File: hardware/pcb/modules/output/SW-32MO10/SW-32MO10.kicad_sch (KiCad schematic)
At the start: 35 parts, among them Q1 NTF2955, Q2 DMN2041L, Q3 DMN2041L, T1 42TL004-RC, U1 SW-32MO, U2 TLV272IS-13

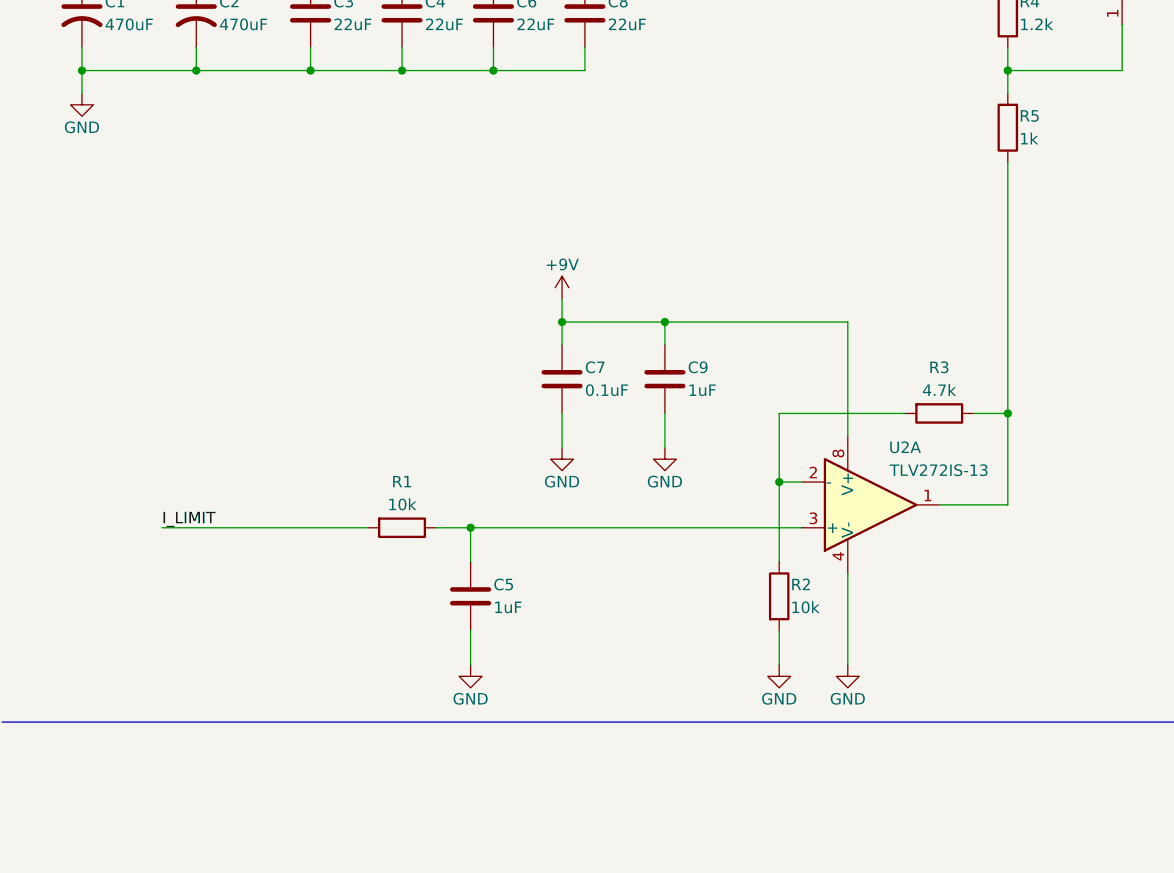
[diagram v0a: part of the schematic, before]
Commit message: update pdf
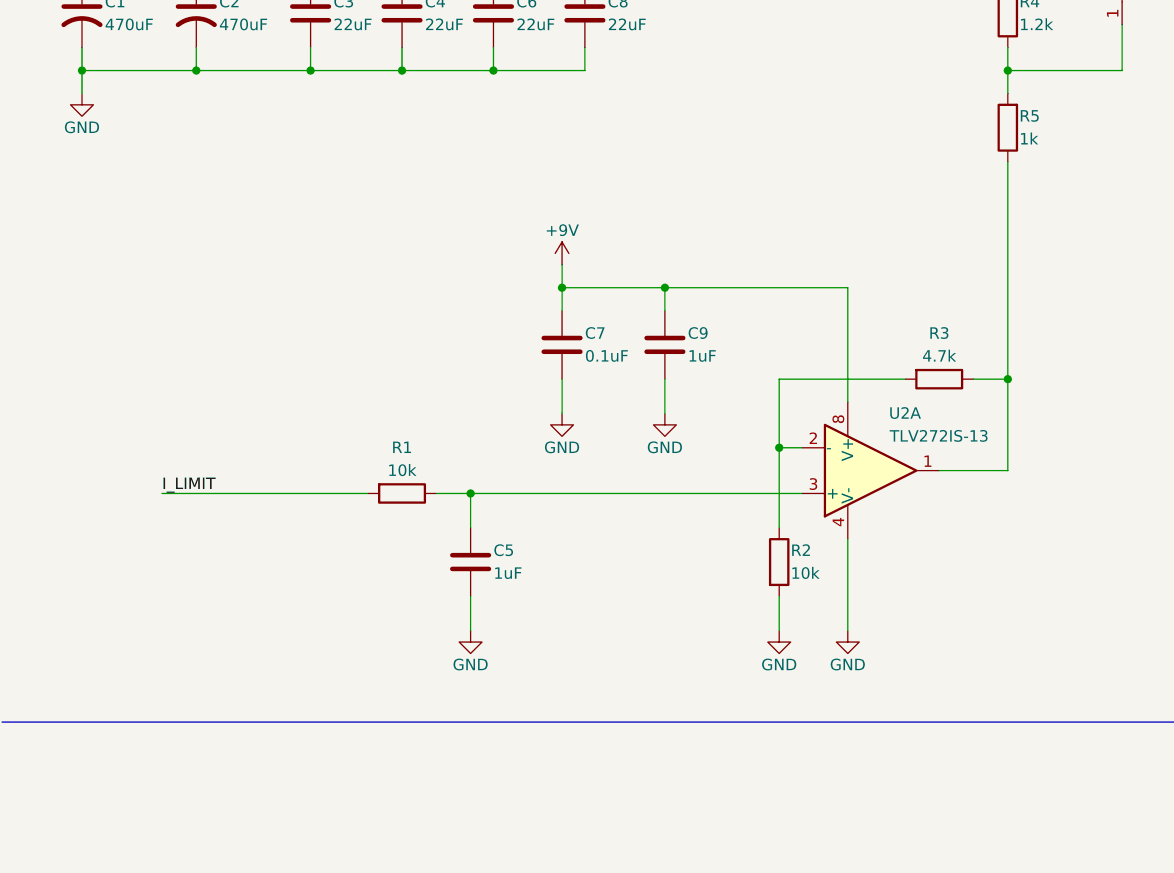
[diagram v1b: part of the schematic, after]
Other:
- moved on the sheet: C5, C7, C9, R1, R2, R3, U2A
